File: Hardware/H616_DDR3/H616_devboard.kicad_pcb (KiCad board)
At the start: 8 copper layers, 50 x 50 mm, 169 parts, among them J1 Micro_SD_Card_Det2, J2 HDMI_D_1.4, J3 USB_C_Receptacle_USB2.0, J4 USB_C_Receptacle_USB2.0, J5 Conn_01x40_Pin, Q1 AO3420_C358680, Q2 AO3401A, Q3 AO3401A, SW1 CK_KMS2xxG, U1 H616, U10 D3V3XA4B10LP, U11 D3V3XA4B10LP, U2 K4B8G1646D, U3 AXP305, U4 SW6206, U6 KLMBG2JETD-B041, U7 AP6256, U8 D3V3XA4B10LP, U9 D3V3XA4B10LP, Y1 24MHz

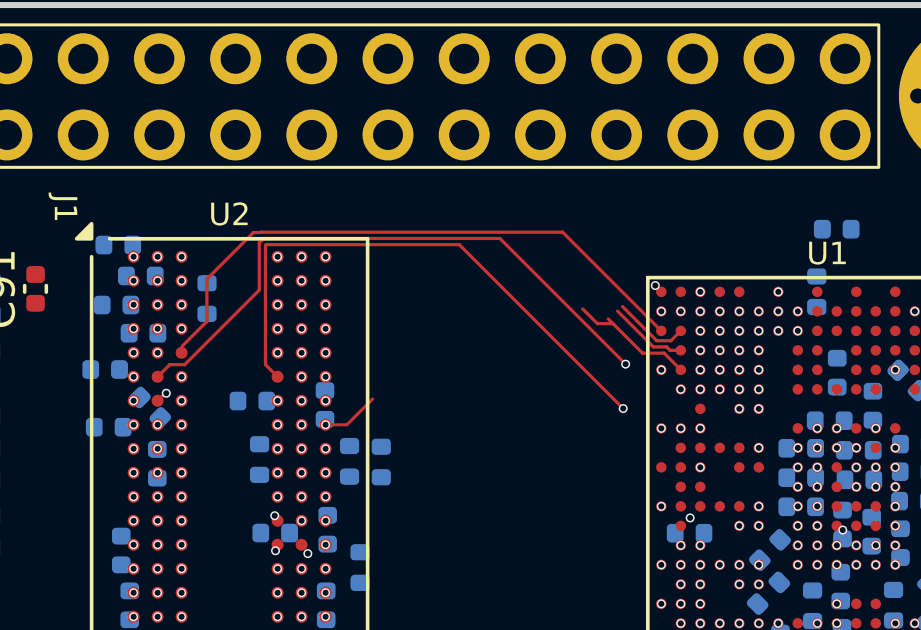
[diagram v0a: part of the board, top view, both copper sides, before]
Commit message: pcb
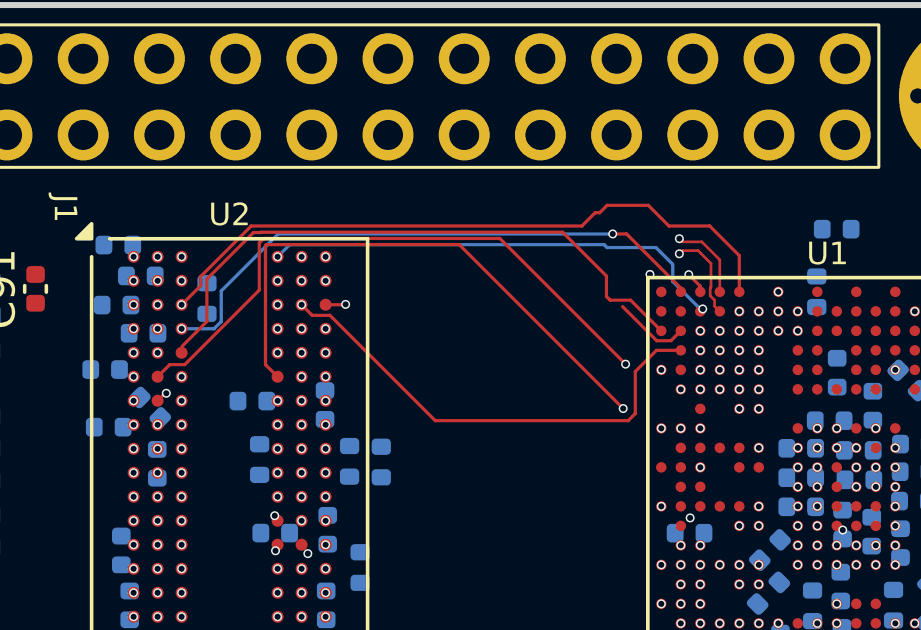
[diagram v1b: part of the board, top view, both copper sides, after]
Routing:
- net /DRAM/DQ9: track 0.00 -> 22.0 mm
- net /DRAM/SDQM0: track 0.00 -> 19.4 mm, vias 1 -> 2
- net /DRAM/SDQS0P: track 0.00 -> 17.6 mm
- net /DRAM/SDQS0N: track 0.00 -> 17.2 mm, vias 1 -> 2
- net /DRAM/DQ12: track 0.00 -> 15.7 mm
- net /DRAM/DQ10: track 2.65 -> 16.0 mm
- net /DRAM/SDQ21: track 4.34 -> 0.00 mm
- net /DRAM/SDQS1P: track 2.92 -> 0.00 mm, vias 2 -> 1
- net /DRAM/SDQS1N: track 2.29 -> 0.00 mm, vias 2 -> 1
- net VCC_DRAM: track 1.93 -> 0.67 mm
- net GND: track 1.34 -> 2.07 mm
